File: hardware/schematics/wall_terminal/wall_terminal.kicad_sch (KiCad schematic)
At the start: 22 parts, among them J1 6P6C, J2 6P6C, J3 Conn_02x12_Odd_Even, J4 Reset, Q1 2N7000, U1 ATtiny13A-P, U2 MAX487E

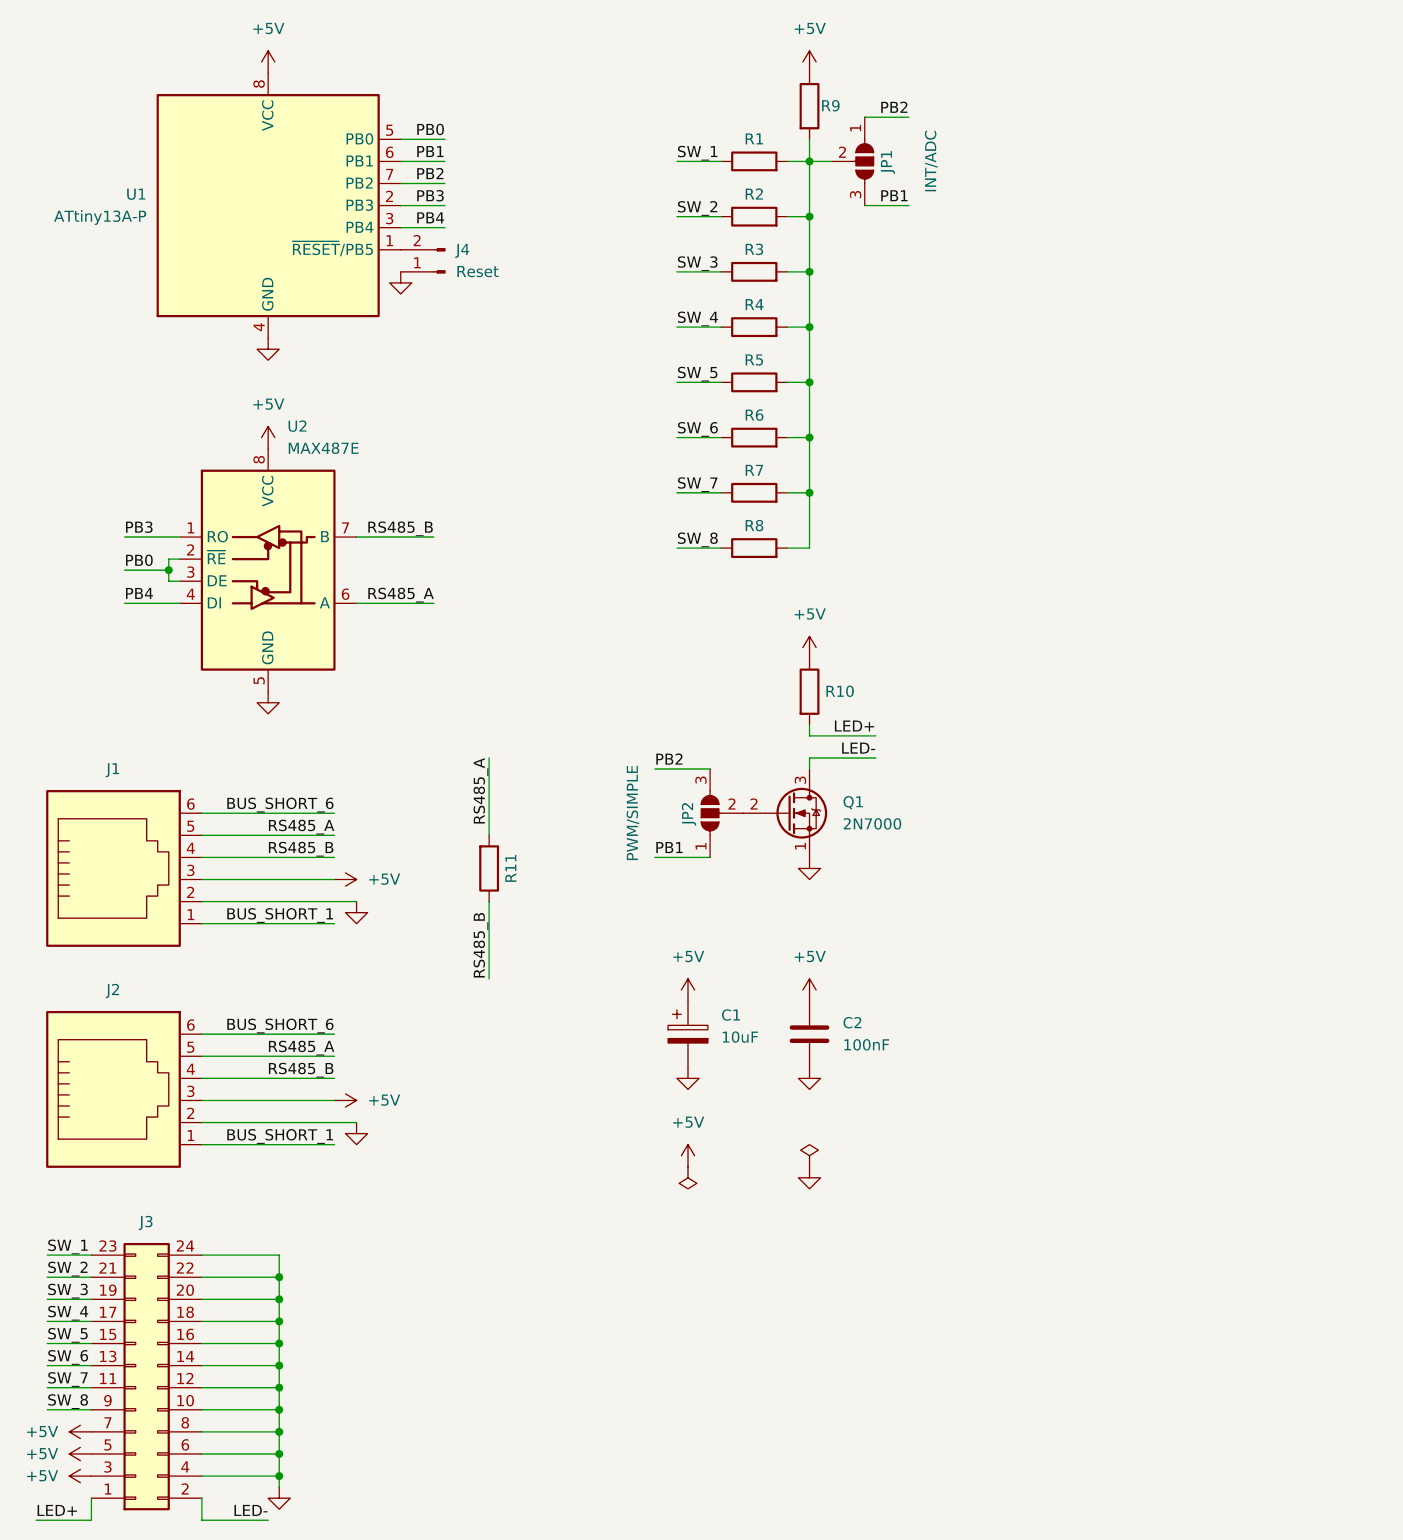
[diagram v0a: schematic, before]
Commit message: !refactor
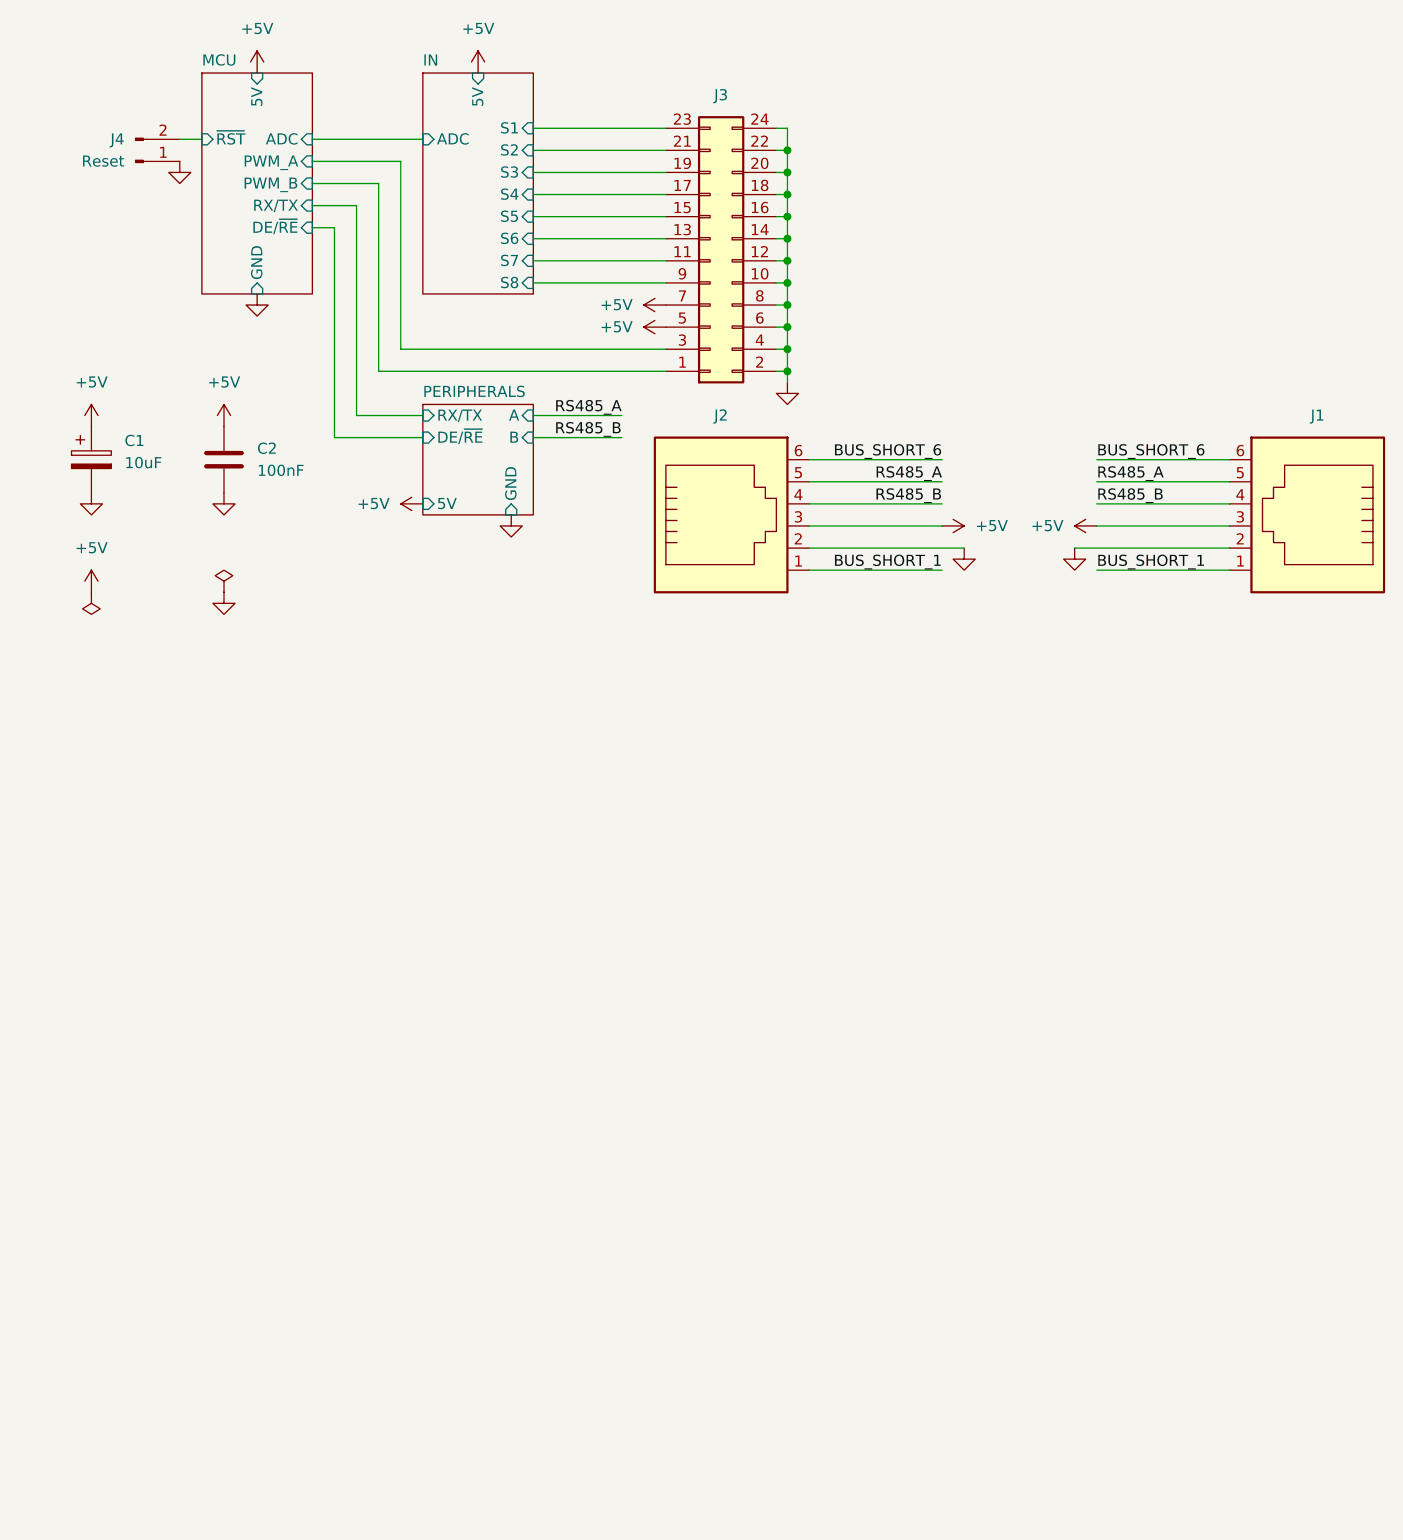
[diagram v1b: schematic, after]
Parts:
- removed JP1: INT/ADC, Jumper:SolderJumper-3_P1.3mm_Open_Pad1.0x1.5mm, symbol Jumper:SolderJumper_3_Open
- removed JP2: PWM/SIMPLE, Jumper:SolderJumper-3_P1.3mm_Open_Pad1.0x1.5mm, symbol Jumper:SolderJumper_3_Open
- removed Q1: 2N7000, Package_TO_SOT_THT:TO-92_Inline, symbol Transistor_FET:2N7000
- removed R1, R10, R2, R3, R4, R5, R6, R7, R8, R9: R, Resistor_THT:R_Axial_DIN0207_L6.3mm_D2.5mm_P2.54mm_Vertical, symbol Device:R
- removed R11: R, Resistor_THT:R_Axial_DIN0207_L6.3mm_D2.5mm_P7.62mm_Horizontal, symbol Device:R
- removed U1: ATtiny13A-P, Package_DIP:DIP-8_W7.62mm_Socket, symbol MCU_Microchip_ATtiny:ATtiny13A-P
- removed U2: MAX487E, Package_DIP:DIP-8_W7.62mm_Socket, symbol Interface_UART:MAX487E
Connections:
- net LED- is gone; now on net GND: J3.2 (Pin_2)
- net +5V: no longer J3.3 (Pin_3)
- net MCU/~{RST}: now reaches J4.2 (Pin_2)
- net LED+ renamed MCU/PWM_B
- net SW_1 renamed IN/S1
- net SW_2 renamed IN/S2
- net SW_3 renamed IN/S3
- net SW_4 renamed IN/S4
- net SW_5 renamed IN/S5
- net SW_6 renamed IN/S6
- net SW_7 renamed IN/S7
- net SW_8 renamed IN/S8
- new net MCU/PWM_A: J3.3 (Pin_3)
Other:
- added sheet IN (in.kicad_sch)
- added sheet MCU (mcu.kicad_sch)
- added sheet PERIPHERALS (peripherals.kicad_sch)
- moved on the sheet: C1, C2, J1, J2, J3
